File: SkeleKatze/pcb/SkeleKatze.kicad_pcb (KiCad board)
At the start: 2 copper layers, 116.3 x 78.3 mm, 6 parts, among them SW1 SW_SPDT

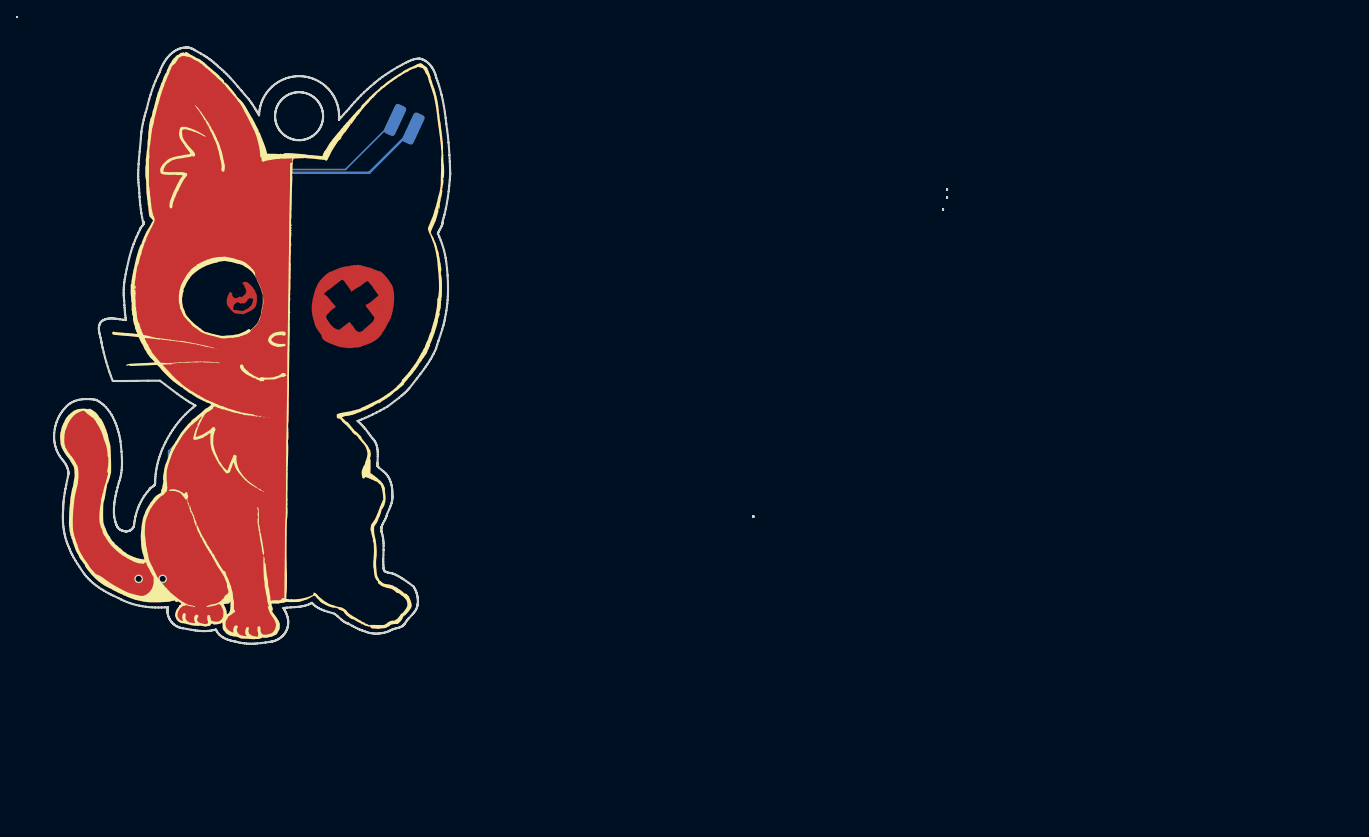
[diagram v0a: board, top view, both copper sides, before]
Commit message: Final cut R 1.0
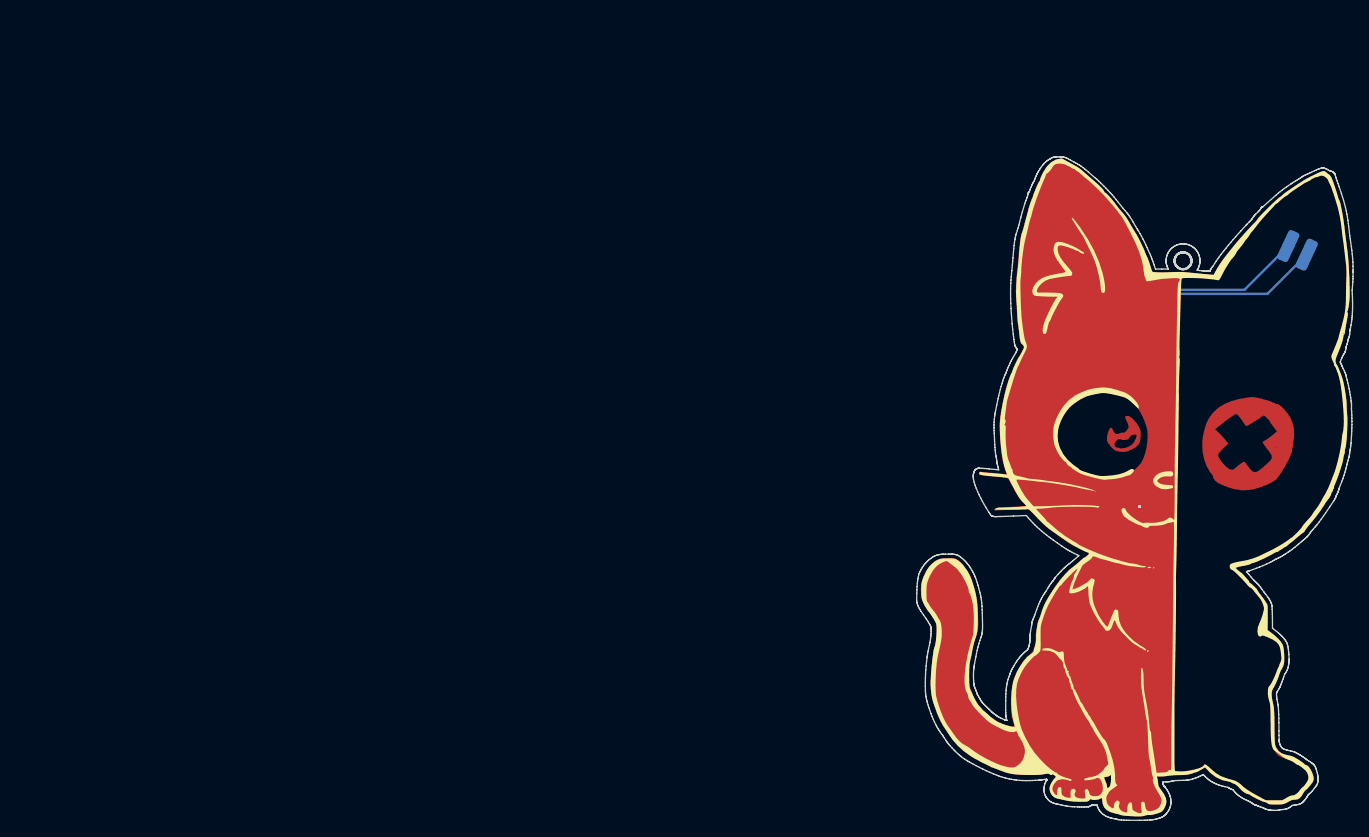
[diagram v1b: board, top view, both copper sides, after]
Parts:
- removed SW1: SW_SPDT, Button_Switch_SMD:SW_SPDT_PCM12
- added SW2: SW_Push, ZAM-Parts:SW_PUSH_SPST_ 1208Yd, B.Cu at (215.0, 87.3)
- Lg1: footprint SkeleKatze-Lib:SkeleKatze-Combined -> SkeleKatze-Lib:SkeleKatze-Merged
- moved Lg1 112.2 mm to (215.0, 77.2)
- moved BT1 110.9 mm to (209.3, 104.6), turned to 0 degrees
- moved D2 110.3 mm to (234.1, 47.0), turned to -115 degrees
- moved Lg2 109.6 mm to (207.1, 43.6)
- moved D1 108.1 mm to (209.8, 59.3), turned to -90 degrees
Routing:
- net Net-(D1-A): track 80.1 -> 64.0 mm
- net GND: track 72.2 -> 81.6 mm
- net Net-(BT1-+): track 40.0 -> 34.8 mm
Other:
- board size 116.3 x 78.3 mm -> 54.5 x 82.9 mm
- board text added: "Schrödingers Katze David Füleki R1.0"
- board text removed: "SkeleKatze R 1.0"
